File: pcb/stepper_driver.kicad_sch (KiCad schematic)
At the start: 20 parts, among them IC1 TMC5240, J3 Conn_01x04_Pin

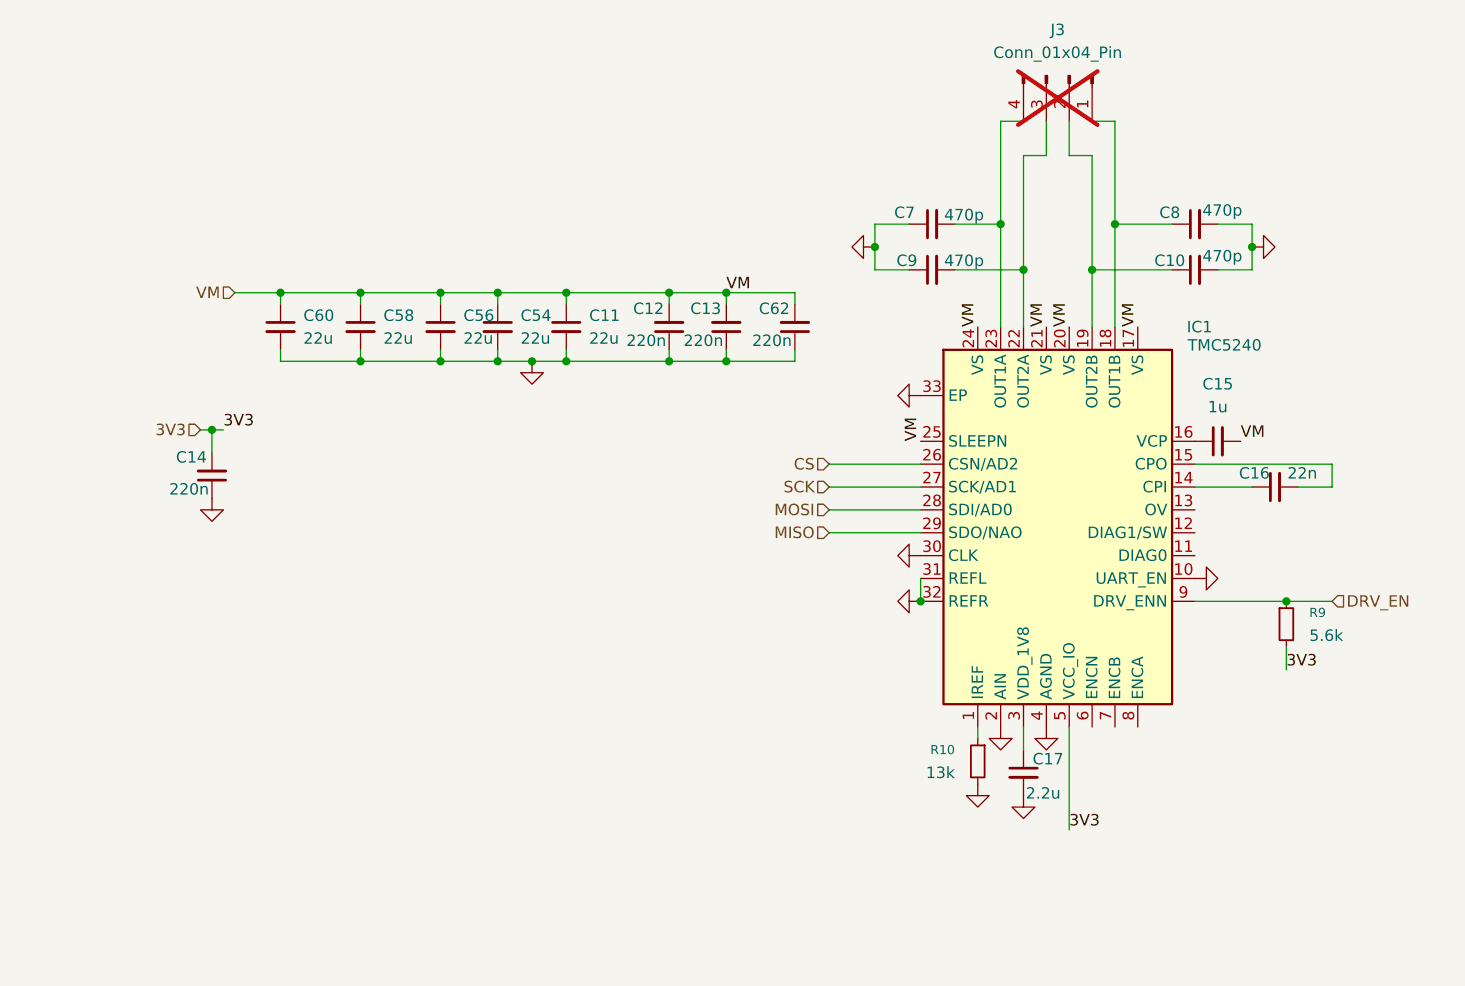
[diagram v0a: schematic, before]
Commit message: PRODUCTION
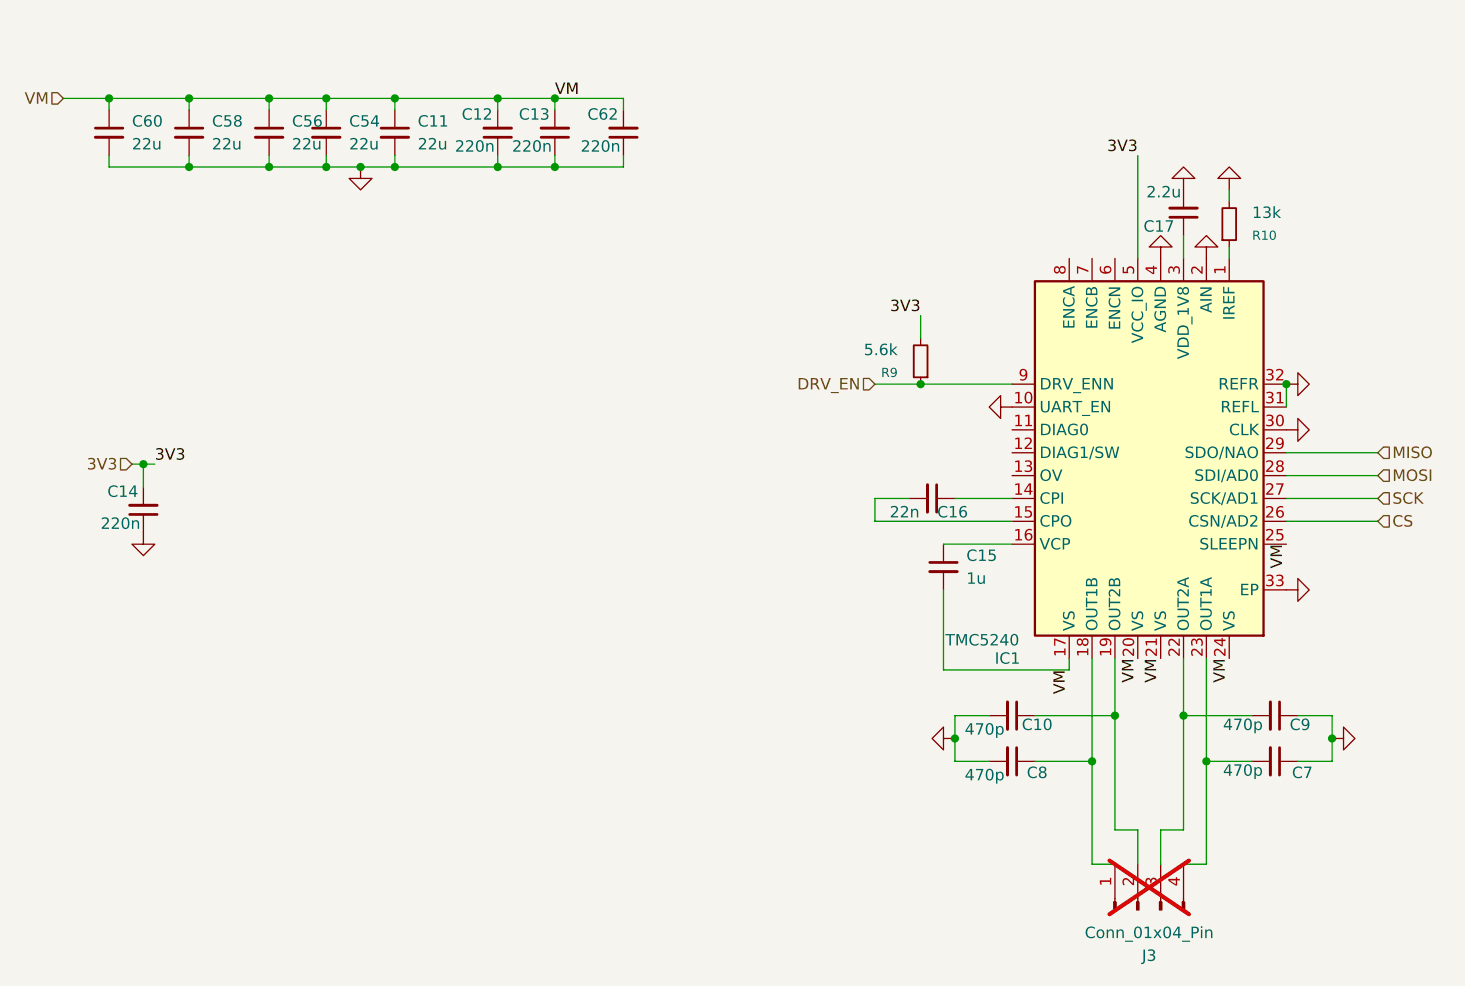
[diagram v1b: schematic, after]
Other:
- moved on the sheet: C10, C11, C12, C13, C14, C15, C16, C17, C54, C56, C58, C60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
